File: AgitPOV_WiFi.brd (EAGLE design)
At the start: 41.2 x 67.6 mm, 41 parts

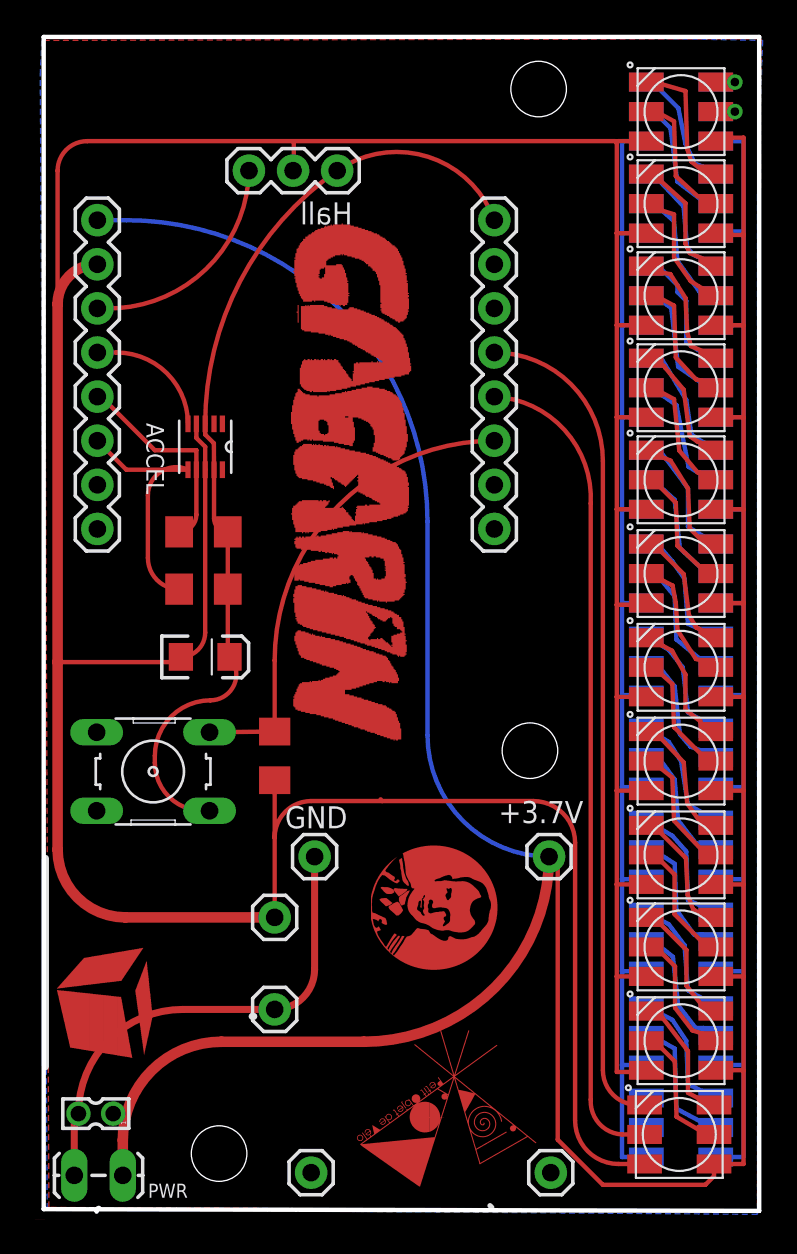
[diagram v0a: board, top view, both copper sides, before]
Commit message: Tout à sa place
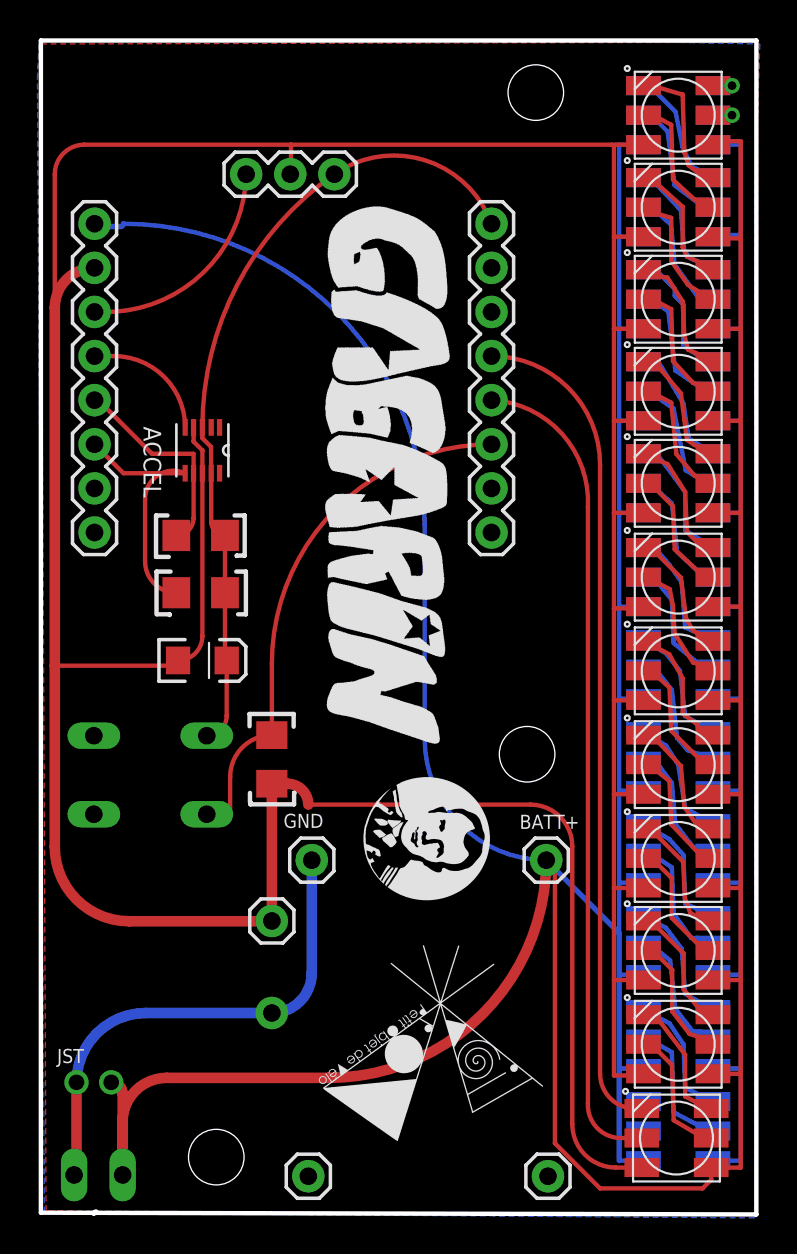
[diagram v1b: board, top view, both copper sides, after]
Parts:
- removed +3.7V: (no value), SparkFun-Connectors:1X01
- removed JP3: SWITCH, SparkFun-Connectors:1X01
- removed JP4: -, SparkFun-Connectors:1X01
- removed PWR: (no value), SparkFun-Connectors:1X02_LOCK_LONGPADS
- added BATT: (no value), SparkFun-Connectors:1X02_LOCK_LONGPADS
- added BATT+: (no value), SparkFun-Connectors:1X01
- added JP-GND: SWITCH, SparkFun-Connectors:1X01
- added JP-GNDE: -, SparkFun-Connectors:1X01
- moved JST 1.81 mm to (3.40, 7.84), flipped to the bottom
- moved WEMOS1 0.26 mm to (26.3, 39.5)
- moved ACCEL 0.26 mm to (9.65, 44.2)
- moved DEL11 0.26 mm to (37.1, 58.2)
- moved FFFFF 0.26 mm to (37.1, 58.2)
- moved GND 0.26 mm to (16.0, 20.6)
- moved PIN0 0.26 mm to (29.6, 2.44)
- moved DEL19 0.26 mm to (37.1, 31.6)
- moved DEL20 0.26 mm to (37.1, 26.3)
- moved DEL5 0.26 mm to (37.1, 26.1)
- moved R3 0.26 mm to (13.7, 26.4)
- moved KK 0.26 mm to (15.8, 2.44)
- moved HALL 0.26 mm to (17.3, 60.1)
- moved DEL1 0.26 mm to (37.0, 4.64)
- moved DEL2 0.26 mm to (37.1, 10.0)
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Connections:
- removed net 5V1: DEL13.1, DEL15.1, DEL16.1, DEL17.1, DEL18.1, DEL19.1, DEL20.1, DEL21.1, DEL22.1, DEL23.1, DEL24.1, FFFFF.1
- removed net GND1: DEL13.6, DEL15.6, DEL16.6, DEL17.6, DEL18.6, DEL19.6, DEL20.6, DEL21.6, DEL22.6, DEL23.6, DEL24.6, FFFFF.6
- removed net N$41: GND.1, JP4.1, JST.2, PWR.2
- new net ENTREEGND: BATT.1, GND.1, JP-GNDE.1, JST.1
- net 5V: now also BATT+.1, BATT.2, DEL13.1, DEL15.1, DEL16.1, DEL17.1, DEL18.1, DEL19.1, DEL20.1, DEL21.1, DEL22.1, DEL23.1, DEL24.1, FFFFF.1, JST.2; no longer +3.7V.1, JST.1, PWR.1
- net GND: now also DEL13.6, DEL15.6, DEL16.6, DEL17.6, DEL18.6, DEL19.6, DEL20.6, DEL21.6, DEL22.6, DEL23.6, DEL24.6, FFFFF.6, JP-GND.1; no longer JP3.1
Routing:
- net 5V: track 191.3 -> 288.4 mm
- net GND1: track 79.3 -> 0.00 mm
- net GND: track 233.8 -> 312.5 mm
- net 5V1: track 75.3 -> 0.00 mm
- net ENTREEGND: track 0.00 -> 28.0 mm
- net N$41: track 27.3 -> 0.00 mm
- net +3.3V: track 51.9 -> 44.7 mm
- net PULLDOWN: track 25.7 -> 28.9 mm
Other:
- board text added: "BATT+"
- board text added: "C1"
- board text added: "R1"
- board text added: "R2"
- board text added: "R3"
- board text removed: "+3.7V"
- board text removed: "/Users/uqam/Documents/logos/logo_ohanda/ohanda_logo.bmp"
